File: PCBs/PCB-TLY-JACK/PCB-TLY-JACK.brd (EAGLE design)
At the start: 57 x 50 mm, 44 parts, among them IC1 ULN2803A, IC2 MCP23017SS, K1 RELAY5VIM03, K2 RELAY5VIM03, K3 RELAY5VIM03, K4 RELAY5VIM03, K5 RELAY5VIM03, K6 RELAY5VIM03, K7 RELAY5VIM03, K8 RELAY5VIM03, X1 DB25F

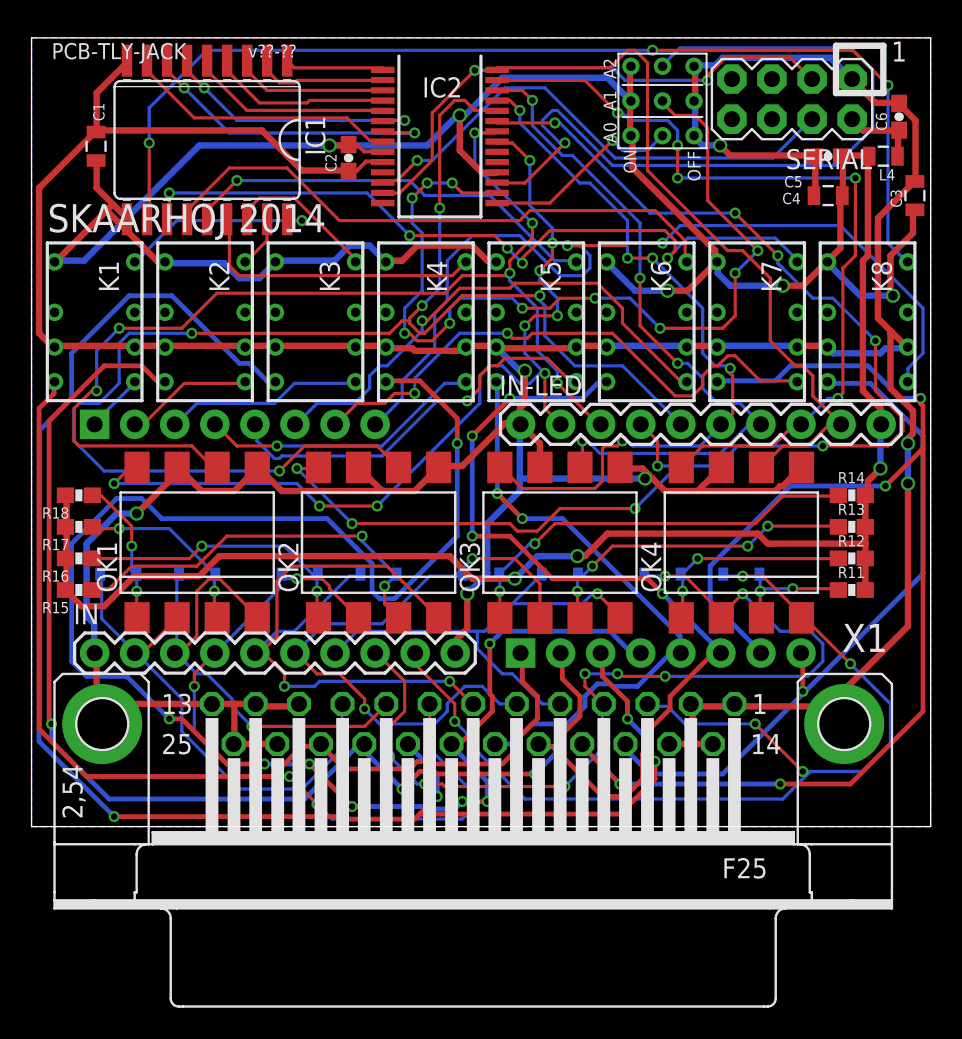
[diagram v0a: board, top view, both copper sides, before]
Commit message: asdf
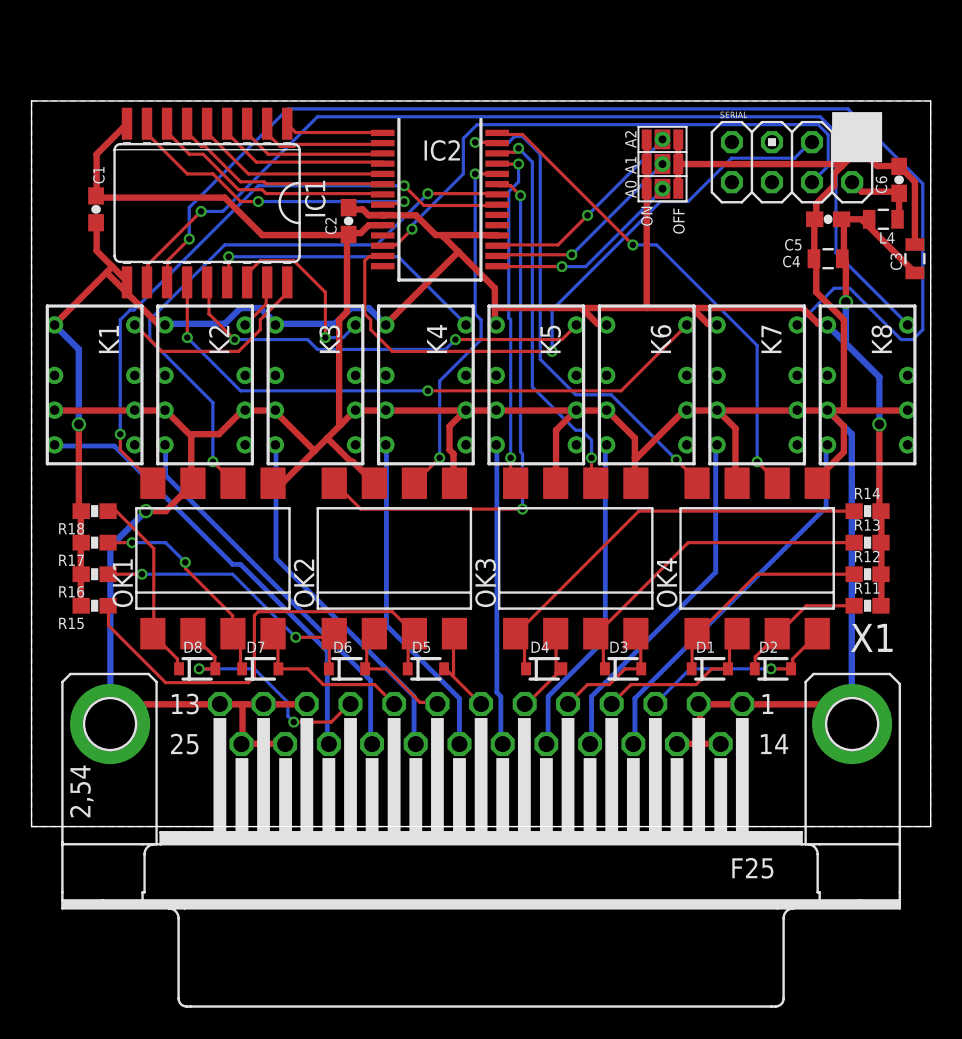
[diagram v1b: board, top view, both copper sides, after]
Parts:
- removed IN, IN-LED: M10", SparkFun:1X10
- removed OUT, OUT-LED: (no value), SparkFun:1X08
- C1: device SparkFun:0805 -> SparkFun:0603-CAP
- SERIAL: value M04X2 -> M04X2M2X4SMALLER; device SparkFun:2X4 -> SKAARHOJ:M2X4SMALLER
- U$19: value 3BITADDR -> 3BITADDRSMALL; device SKAARHOJ:3BITADDR -> SKAARHOJ:3BITADDR_SMALL
- moved D8 7.81 mm to (10.5, 10.0), flipped to the top
- moved D3 7.21 mm to (37.5, 10.0), flipped to the top
- moved D4 7.21 mm to (32.5, 10.0), flipped to the top
- moved D7 7.21 mm to (14.5, 10.0), flipped to the top
- moved D1 6.71 mm to (43.0, 10.0), flipped to the top
- moved D5 6.71 mm to (25.0, 10.0), flipped to the top
- moved D6 6.71 mm to (20.0, 10.0), flipped to the top
- moved D2 6.32 mm to (47.0, 10.0), flipped to the top
- moved C1 4.00 mm to (4.09, 39.1)
- moved C2 4.00 mm to (20.1, 38.4)
- moved C3 4.00 mm to (56.0, 36.0)
- moved C4 4.00 mm to (50.5, 36.0)
- moved C5 4.00 mm to (50.5, 38.5)
- moved C6 4.00 mm to (55.0, 41.0)
- moved IC1 4.00 mm to (11.1, 39.5)
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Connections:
- net 5V: now also U$19.H0; no longer IN-LED.10, U$19.H3
- net A0: now also U$19.AS0
- net A1: now also U$19.AS1
- net A2: now also U$19.AS2
- net GND: now also U$19.L0; no longer IN-LED.1, IN.1, IN.10, U$19.L3
- net IN1: no longer IN-LED.2
- net IN2: no longer IN-LED.3
- net IN3: no longer IN-LED.4
- net IN4: no longer IN-LED.5
- net IN5: no longer IN-LED.6
- net IN6: no longer IN-LED.7
- net IN7: no longer IN-LED.8
- net IN8: no longer IN-LED.9
- net N$1: no longer OUT.1
- net N$10: no longer OUT.3
- net N$14: no longer OUT.4
- net N$18: no longer OUT.5
- net N$22: no longer OUT.6
- net N$26: no longer OUT.7
- net N$30: no longer OUT.8
- net N$49: no longer IN.2
- net N$55: no longer IN.6
- net N$6: no longer OUT.2
- net N$60: no longer IN.3
- net N$61: no longer IN.4
- net N$62: no longer IN.5
- net N$64: no longer IN.7
- net N$65: no longer IN.8
- net N$66: no longer IN.9
- net O1: no longer OUT-LED.1
- net O2: no longer OUT-LED.2
- net O3: no longer OUT-LED.3
- net O4: no longer OUT-LED.4
- net O5: no longer OUT-LED.5
- net O6: no longer OUT-LED.6
- net O7: no longer OUT-LED.7
- net O8: no longer OUT-LED.8
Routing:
- net 5V: track 230.5 -> 143.5 mm, vias 8 -> 3
- net N$14: track 104.7 -> 20.9 mm, vias 8 -> 0
- net N$10: track 99.3 -> 22.7 mm, vias 4 -> 0
- net IN4: track 91.1 -> 22.9 mm, vias 5 -> 2
- net N$26: track 82.1 -> 22.3 mm, vias 4 -> 0
- net GND: track 302.7 -> 246.0 mm, vias 7 -> 1
- net O8: track 56.0 -> 0.00 mm, vias 2 -> 0
- net N$66: track 65.7 -> 12.5 mm, vias 5 -> 1
- net IN3: track 85.0 -> 34.3 mm, vias 9 -> 2
- net N$6: track 74.9 -> 24.4 mm, vias 4 -> 0
- net N$65: track 60.0 -> 10.8 mm, vias 8 -> 0
- net A1: track 57.3 -> 12.9 mm, vias 10 -> 1
- net N$61: track 46.8 -> 7.93 mm, vias 5 -> 0
- net O7: track 36.2 -> 0.00 mm, vias 2 -> 0
- net N$62: track 42.1 -> 6.01 mm, vias 2 -> 0
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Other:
- board size 57 x 50 mm -> 57 x 46 mm
- board text added: "PCB-TLY-JACK, v02-16 SKAARHOJ"
- board text removed: "1"
- board text removed: "PCB-TLY-JACK"
- board text removed: "SKAARHOJ 2014"
- board text removed: "v??-??"
